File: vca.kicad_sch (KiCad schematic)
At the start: 66 parts, among them J1 Signal 1, J2 Signal 2, J3 CV 1, J4 CV 2, J5 Out 1, J6 Out 2, J7 Conn_02x05_Odd_Even, Q1 BCM847, Q2 BC547C, U1 TL074

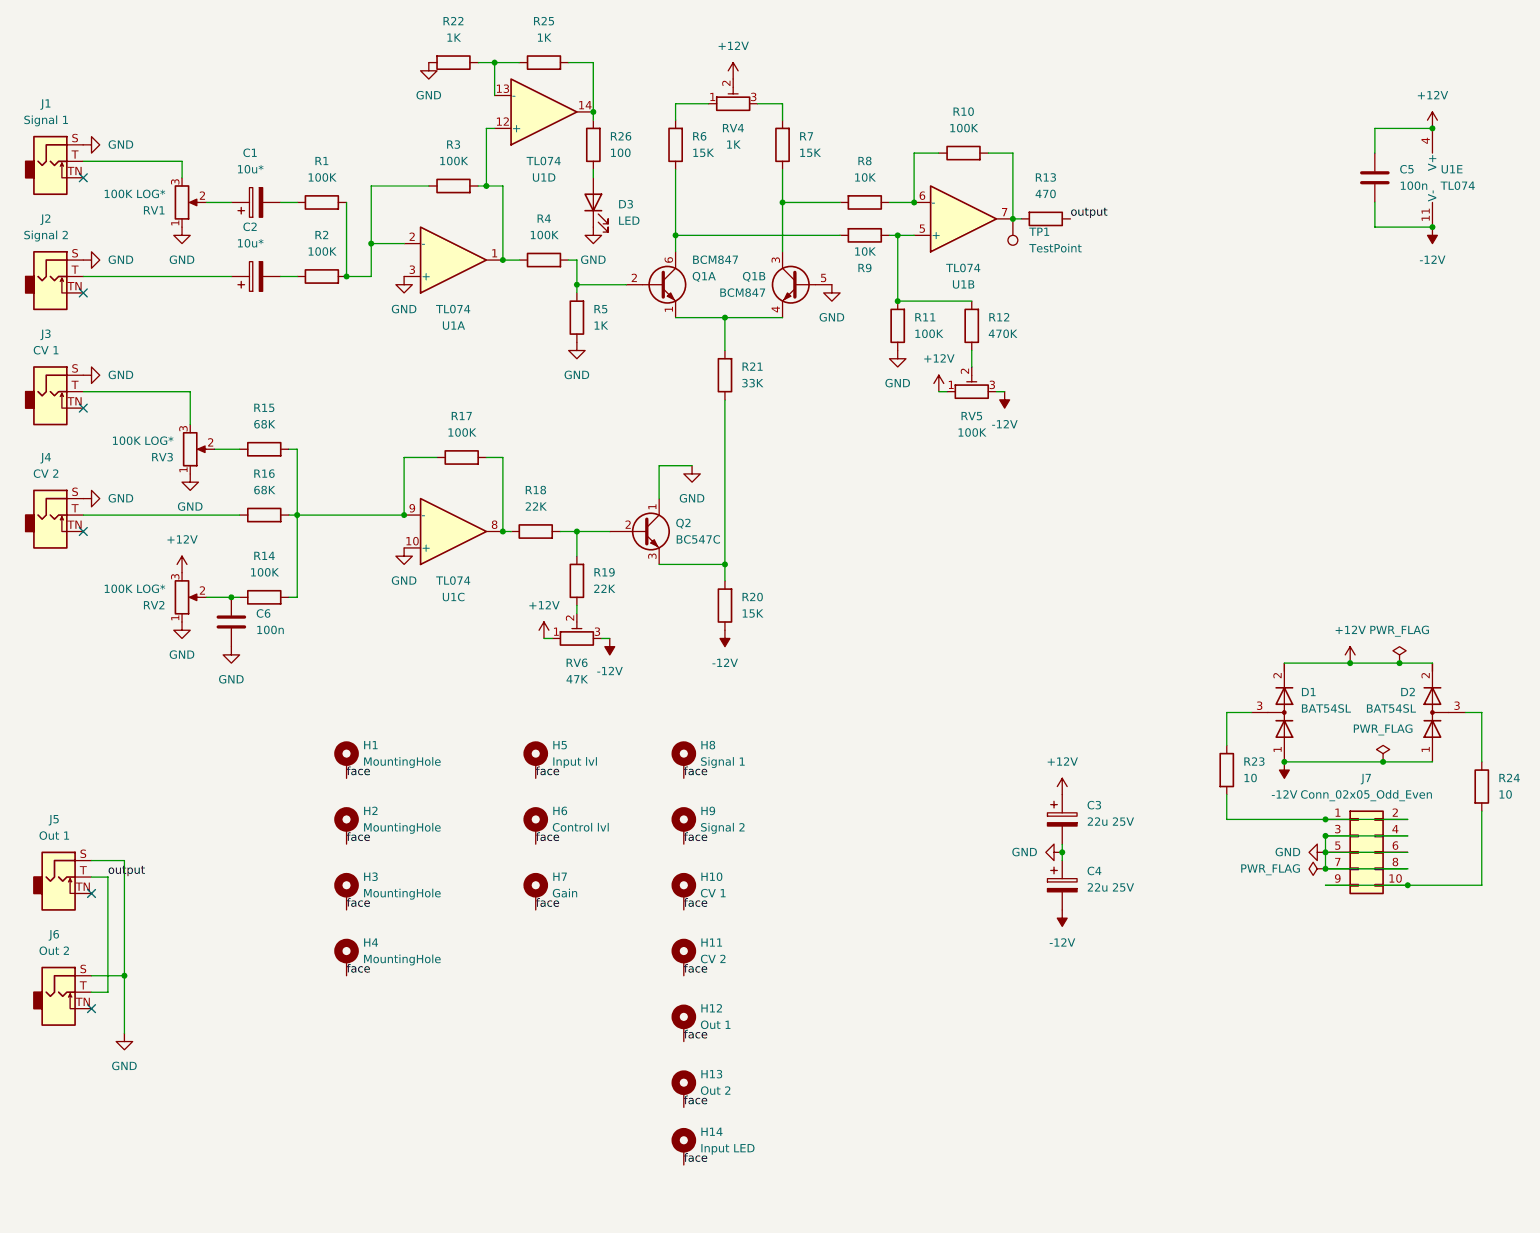
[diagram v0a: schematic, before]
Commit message: v2 ready
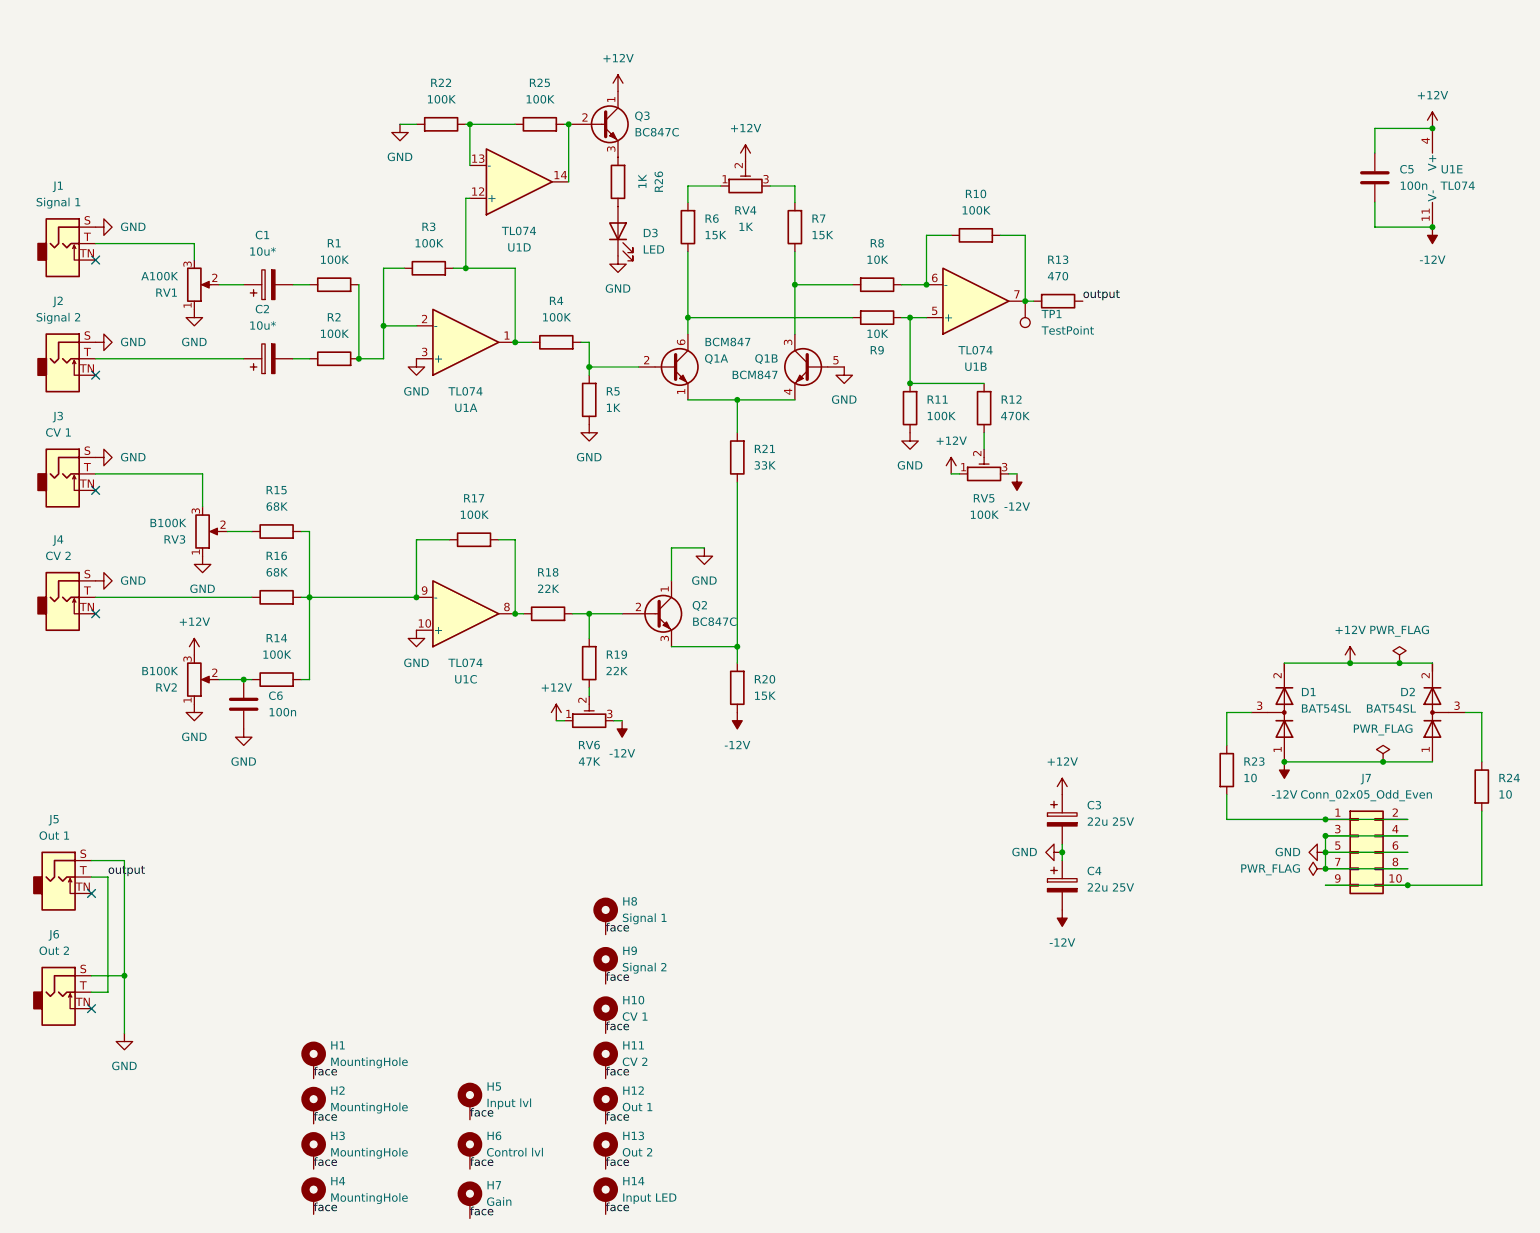
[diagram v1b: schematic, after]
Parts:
- removed Q2: BC547C, Package_TO_SOT_THT:TO-92L_Inline, symbol Device:Q_NPN_CBE
- added Q2, Q3: BC847C, Package_TO_SOT_SMD:SOT-23-3, symbol eurorack:BC547
- H10, H11: footprint eurorack:Mech-AudioJack-Hole -> eurorack:Mech-AudioJack-Hole-Input-CV
- H14: footprint eurorack:Mech-LED-Hole-4mm -> eurorack:Mech-LED-Hole-3mm-Bezel
- H8, H9: footprint eurorack:Mech-AudioJack-Hole -> eurorack:Mech-AudioJack-Hole-Input
- R22, R25: value 1K -> 100K
- R26: value 100 -> 1K
- RV1: value 100K LOG* -> A100K
- RV2, RV3: value 100K LOG* -> B100K
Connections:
- net +12V: now also Q3.1 (C)
- net GND: now also Q2.1 (C)
- net at R18.2, R19.2: now also Q2.2 (B)
- net at R25.2, U1.14: now also Q3.2 (B); no longer R26.2
- net at R20.2, R21.1: now also Q2.3 (E)
- new net: Q3.3 (E), R26.2
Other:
- moved on the sheet: C1, C2, C6, D3, H1, H10, H11, H12, H13, H14, H2, H3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
